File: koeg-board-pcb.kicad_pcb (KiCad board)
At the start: 2 copper layers, 10 parts, among them SW1 SW_Push_45deg, SW2 SW_Push_45deg, SW3 SW_Push_45deg, SW4 SW_Push_45deg, SW5 SW_Push_45deg, SW6 SW_Push_45deg, SW7 SW_Push_45deg, SW8 SW_Push_45deg, SW9 SW_Push_45deg, U1 STM32F730V8Tx

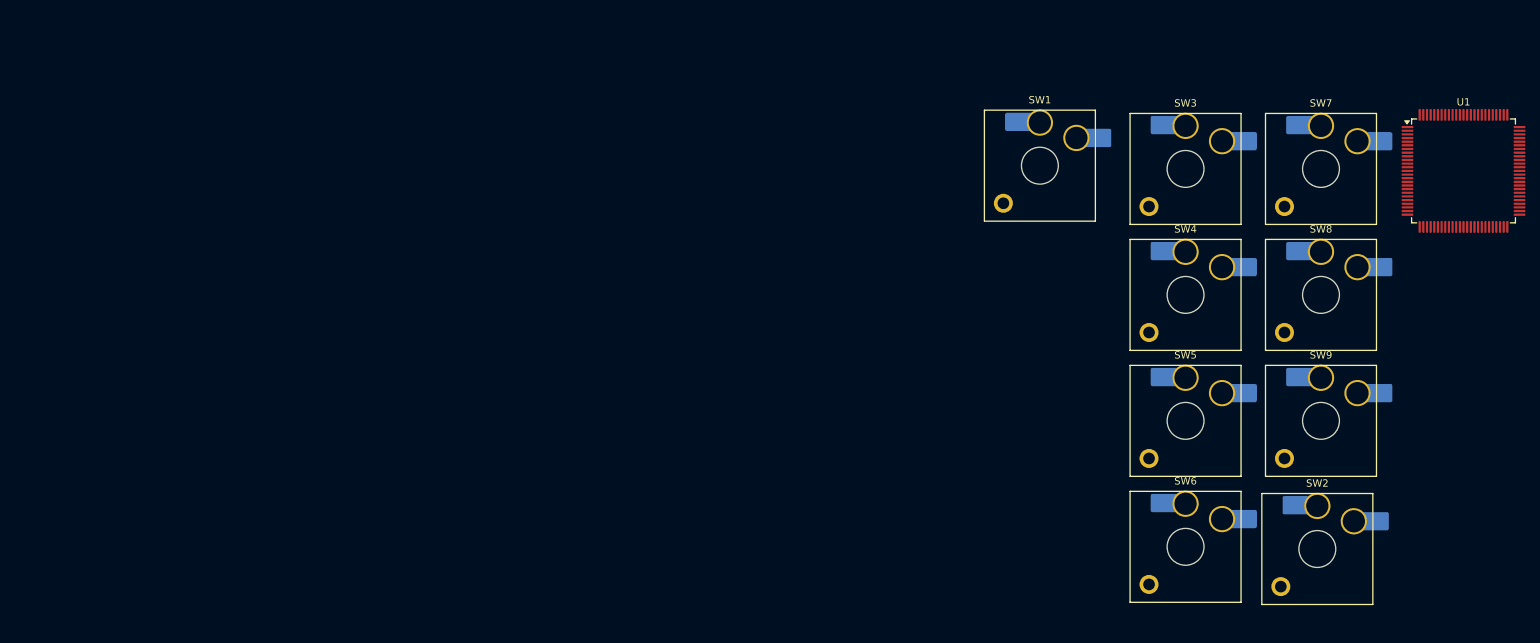
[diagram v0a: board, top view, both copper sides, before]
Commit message: before auto route
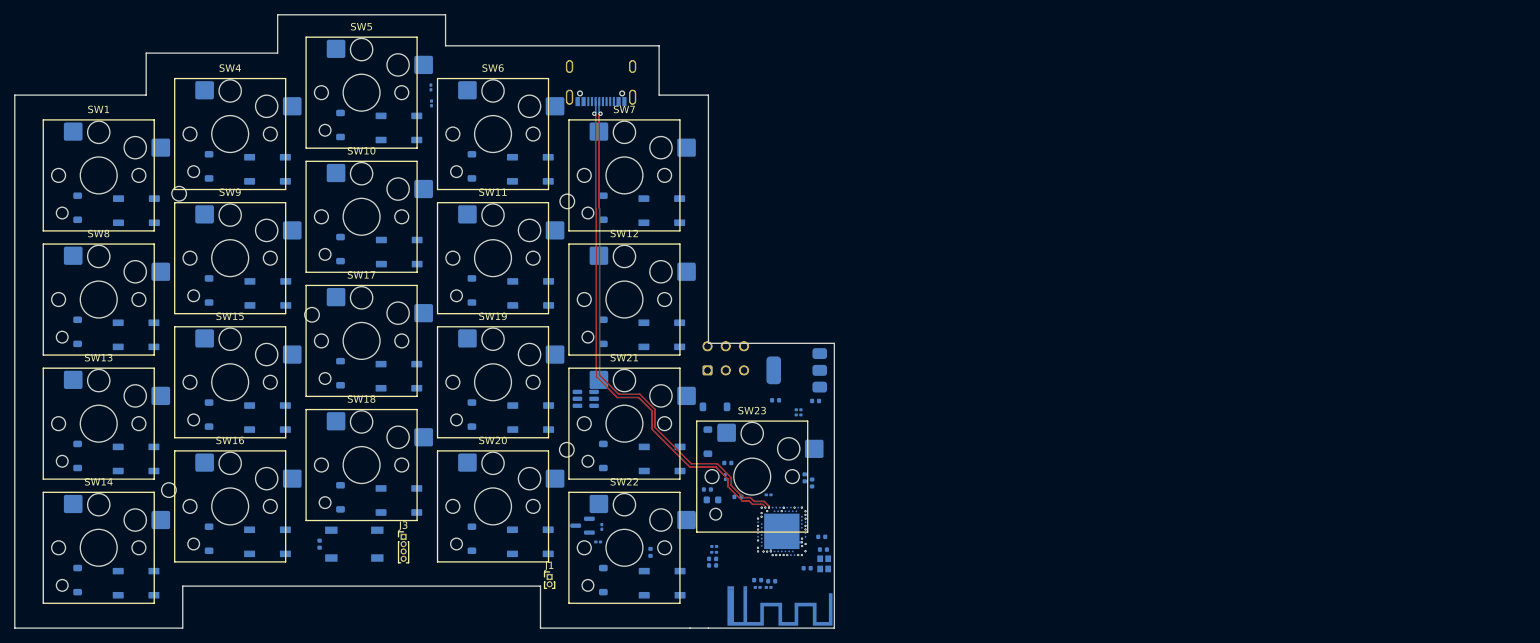
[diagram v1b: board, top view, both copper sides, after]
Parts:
- added AE1: PCB_Antenna, pcb_ant:pcb_antenna, B.Cu at (132.9, 122.5)
- added C1: 12pF, Capacitor_SMD:C_0402_1005Metric, B.Cu at (142.1, 119.5)
- added C10: 1pF, Capacitor_SMD:C_0402_1005Metric, B.Cu at (137.3, 121.3)
- added C11: 1.2pF, Capacitor_SMD:C_0402_1005Metric, B.Cu at (135.3, 121.1)
- added C12: 4.7uF, Capacitor_SMD:C_0402_1005Metric, B.Cu at (128.5, 108.7)
- added C13: 4.7uF, Capacitor_SMD:C_0402_1005Metric, B.Cu at (141.8, 107.1)
- added C14: 1uF, Capacitor_SMD:C_0402_1005Metric, B.Cu at (143.3, 96.6)
- added C15: 1uF, Capacitor_SMD:C_0402_1005Metric, B.Cu at (137.8, 96.5)
- added C16: 100nF, Capacitor_SMD:C_0402_1005Metric, B.Cu at (75.3, 116.2)
- added C2: 12pF, Capacitor_SMD:C_0402_1005Metric, B.Cu at (144.3, 116.9)
- added C3: 100nF, Capacitor_SMD:C_0402_1005Metric, B.Cu at (131.3, 105.1)
- added C4: 100pF, Capacitor_SMD:C_0402_1005Metric, B.Cu at (142.8, 107.8)
- added C5: 1uF, Capacitor_SMD:C_0402_1005Metric, B.Cu at (129.2, 119.1)
- added C6: 47nF, Capacitor_SMD:C_0402_1005Metric, B.Cu at (129.2, 118.2)
- added C7: 820pF, Capacitor_SMD:C_0402_1005Metric, B.Cu at (144.1, 115.2)
- added C8: 4.7uF, Capacitor_SMD:C_0402_1005Metric, B.Cu at (132.6, 109.7)
- added C9: 4.7uF, Capacitor_SMD:C_0402_1005Metric, B.Cu at (120.7, 117.3)
- added D1: 1N5819, Diode_SMD:D_SOD-123, B.Cu at (42.2, 70.1)
- added D10: 1N5819, Diode_SMD:D_SOD-123, B.Cu at (96.2, 81.4)
- added D11: 1N5819, Diode_SMD:D_SOD-123, B.Cu at (114.2, 87.1)
- added D12: 1N5819, Diode_SMD:D_SOD-123, B.Cu at (42.2, 104.1)
- added D13: 1N5819, Diode_SMD:D_SOD-123, B.Cu at (42.2, 121.1)
- added D14: 1N5819, Diode_SMD:D_SOD-123, B.Cu at (60.2, 98.4)
- added D15: 1N5819, Diode_SMD:D_SOD-123, B.Cu at (60.2, 115.4)
- added D16: 1N5819, Diode_SMD:D_SOD-123, B.Cu at (78.2, 92.8)
- added D17: 1N5819, Diode_SMD:D_SOD-123, B.Cu at (78.2, 109.8)
- added D18: 1N5819, Diode_SMD:D_SOD-123, B.Cu at (96.2, 98.4)
- added D19: 1N5819, Diode_SMD:D_SOD-123, B.Cu at (96.2, 115.4)
- added D2: 1N5819, Diode_SMD:D_SOD-123, B.Cu at (129.5, 97.4)
- added D20: 1N5819, Diode_SMD:D_SOD-123, B.Cu at (114.2, 104.1)
- added D21: 1N5819, Diode_SMD:D_SOD-123, B.Cu at (114.2, 121.1)
- added D22: 1N5819, Diode_SMD:D_SOD-123, B.Cu at (128.5, 102.1)
- added D23: WS2812B-2020, LED_SMD:LED_WS2812B_PLCC4_5.0x5.0mm_P3.2mm, B.Cu at (122.3, 121.5)
- added D24: WS2812B-2020, LED_SMD:LED_WS2812B_PLCC4_5.0x5.0mm_P3.2mm, B.Cu at (104.2, 115.9)
- added D25: WS2812B-2020, LED_SMD:LED_WS2812B_PLCC4_5.0x5.0mm_P3.2mm, B.Cu at (86.2, 110.2)
- added D26: WS2812B-2020, LED_SMD:LED_WS2812B_PLCC4_5.0x5.0mm_P3.2mm, B.Cu at (68.2, 115.9)
- added D27: WS2812B-2020, LED_SMD:LED_WS2812B_PLCC4_5.0x5.0mm_P3.2mm, B.Cu at (50.2, 121.5)
- added D28: WS2812B-2020, LED_SMD:LED_WS2812B_PLCC4_5.0x5.0mm_P3.2mm, B.Cu at (122.3, 104.5)
- added D29: WS2812B-2020, LED_SMD:LED_WS2812B_PLCC4_5.0x5.0mm_P3.2mm, B.Cu at (104.3, 98.8)
- added D3: 1N5819, Diode_SMD:D_SOD-123, B.Cu at (60.2, 64.4)
- added D30: WS2812B-2020, LED_SMD:LED_WS2812B_PLCC4_5.0x5.0mm_P3.2mm, B.Cu at (86.2, 93.2)
- added D31: WS2812B-2020, LED_SMD:LED_WS2812B_PLCC4_5.0x5.0mm_P3.2mm, B.Cu at (68.2, 98.8)
- added D32: WS2812B-2020, LED_SMD:LED_WS2812B_PLCC4_5.0x5.0mm_P3.2mm, B.Cu at (50.2, 104.5)
- added D33: WS2812B-2020, LED_SMD:LED_WS2812B_PLCC4_5.0x5.0mm_P3.2mm, B.Cu at (122.2, 87.5)
- added D34: WS2812B-2020, LED_SMD:LED_WS2812B_PLCC4_5.0x5.0mm_P3.2mm, B.Cu at (104.3, 81.8)
- added D35: WS2812B-2020, LED_SMD:LED_WS2812B_PLCC4_5.0x5.0mm_P3.2mm, B.Cu at (86.3, 76.2)
- added D36: WS2812B-2020, LED_SMD:LED_WS2812B_PLCC4_5.0x5.0mm_P3.2mm, B.Cu at (68.3, 81.8)
- added D37: WS2812B-2020, LED_SMD:LED_WS2812B_PLCC4_5.0x5.0mm_P3.2mm, B.Cu at (50.2, 87.5)
- added D38: WS2812B-2020, LED_SMD:LED_WS2812B_PLCC4_5.0x5.0mm_P3.2mm, B.Cu at (122.2, 70.5)
- added D39: WS2812B-2020, LED_SMD:LED_WS2812B_PLCC4_5.0x5.0mm_P3.2mm, B.Cu at (104.2, 64.8)
- added D4: 1N5819, Diode_SMD:D_SOD-123, B.Cu at (78.2, 58.8)
- added D40: WS2812B-2020, LED_SMD:LED_WS2812B_PLCC4_5.0x5.0mm_P3.2mm, B.Cu at (86.2, 59.2)
- added D41: WS2812B-2020, LED_SMD:LED_WS2812B_PLCC4_5.0x5.0mm_P3.2mm, B.Cu at (68.2, 64.8)
- added D42: WS2812B-2020, LED_SMD:LED_WS2812B_PLCC4_5.0x5.0mm_P3.2mm, B.Cu at (50.3, 70.5)
- added D5: 1N5819, Diode_SMD:D_SOD-123, B.Cu at (96.2, 64.4)
- added D6: 1N5819, Diode_SMD:D_SOD-123, B.Cu at (114.2, 70.1)
- added D7: 1N5819, Diode_SMD:D_SOD-123, B.Cu at (42.2, 87.1)
- added D8: 1N5819, Diode_SMD:D_SOD-123, B.Cu at (60.2, 81.4)
- added D9: 1N5819, Diode_SMD:D_SOD-123, B.Cu at (78.2, 75.8)
- added F1: 500mA, Fuse:Fuse_0603_1608Metric, B.Cu at (129.2, 110.1)
- added H1: MountingHole, MountingHole:MountingHole_2mm, B.Cu at (56.1, 68.2)
- added H2: MountingHole, MountingHole:MountingHole_2mm, B.Cu at (74.3, 84.8)
- added H3: MountingHole, MountingHole:MountingHole_2mm, B.Cu at (109.2, 103.3)
- added H4: MountingHole, MountingHole:MountingHole_2mm, B.Cu at (54.7, 108.8)
- added H5: MountingHole, MountingHole:MountingHole_2mm, B.Cu at (109.3, 69.2)
- added J1: Conn_01x02, Connector_PinHeader_1.00mm:PinHeader_1x02_P1.00mm_Vertical, F.Cu at (106.8, 120.7)
- added J2: USB_C_Receptacle_USB2.0_14P, Connector_USB:USB_C_Receptacle_G-Switch_GT-USB-7010ASV, B.Cu at (113.9, 51.8)
- added J3: SWD_Connector, Connector_PinHeader_1.00mm:PinHeader_1x04_P1.00mm_Vertical, F.Cu at (86.8, 115.2)
- added L1: 10uH, Inductor_SMD:L_0201_0603Metric, B.Cu at (129.4, 116.5)
- added L2: 15nH, Inductor_SMD:L_0201_0603Metric, B.Cu at (129.4, 117.3)
- added L3: 10uH, Inductor_SMD:L_0201_0603Metric, B.Cu at (130.9, 107.0)
- added L4: 4.7nH, Inductor_SMD:L_0201_0603Metric, B.Cu at (136.8, 122.1)
- added L5: 2.2nH, Inductor_SMD:L_0201_0603Metric, B.Cu at (135.3, 122.1)
- added Q1: BSS138, Package_TO_SOT_SMD:SOT-23, B.Cu at (111.4, 113.7)
- added R1: 5.1k, Resistor_SMD:R_0201_0603Metric, B.Cu at (90.6, 53.6)
- added R2: 5.1k, Resistor_SMD:R_0201_0603Metric, B.Cu at (90.7, 55.8)
- added R3: 2M, Resistor_SMD:R_0201_0603Metric, B.Cu at (140.9, 98.5)
- added R4: 810K, Resistor_SMD:R_0201_0603Metric, B.Cu at (141.0, 97.8)
- added R5: 10K, Resistor_SMD:R_0201_0603Metric, B.Cu at (114.0, 113.8)
- added R6: 10K, Resistor_SMD:R_0201_0603Metric, B.Cu at (113.5, 115.9)
- added R7: 100K, Resistor_SMD:R_0201_0603Metric, B.Cu at (136.8, 109.4)
- added SW10: SW_Push, PCM_Switch_Keyboard_Hotswap_Kailh:SW_Hotswap_Kailh_Choc_V1V2_1.00u, F.Cu at (81.1, 71.3)
- added SW11: SW_Push, PCM_Switch_Keyboard_Hotswap_Kailh:SW_Hotswap_Kailh_Choc_V1V2_1.00u, F.Cu at (99.1, 77.0)
- added SW12: SW_Push, PCM_Switch_Keyboard_Hotswap_Kailh:SW_Hotswap_Kailh_Choc_V1V2_1.00u, F.Cu at (117.1, 82.7)
- added SW13: SW_Push, PCM_Switch_Keyboard_Hotswap_Kailh:SW_Hotswap_Kailh_Choc_V1V2_1.00u, F.Cu at (45.1, 99.7)
- added SW14: SW_Push, PCM_Switch_Keyboard_Hotswap_Kailh:SW_Hotswap_Kailh_Choc_V1V2_1.00u, F.Cu at (45.1, 116.7)
- added SW15: SW_Push, PCM_Switch_Keyboard_Hotswap_Kailh:SW_Hotswap_Kailh_Choc_V1V2_1.00u, F.Cu at (63.1, 94.0)
- added SW16: SW_Push, PCM_Switch_Keyboard_Hotswap_Kailh:SW_Hotswap_Kailh_Choc_V1V2_1.00u, F.Cu at (63.1, 111.0)
- added SW17: SW_Push, PCM_Switch_Keyboard_Hotswap_Kailh:SW_Hotswap_Kailh_Choc_V1V2_1.00u, F.Cu at (81.1, 88.3)
- added SW18: SW_Push, PCM_Switch_Keyboard_Hotswap_Kailh:SW_Hotswap_Kailh_Choc_V1V2_1.00u, F.Cu at (81.1, 105.3)
- added SW19: SW_Push, PCM_Switch_Keyboard_Hotswap_Kailh:SW_Hotswap_Kailh_Choc_V1V2_1.00u, F.Cu at (99.1, 94.0)
- added SW20: SW_Push, PCM_Switch_Keyboard_Hotswap_Kailh:SW_Hotswap_Kailh_Choc_V1V2_1.00u, F.Cu at (99.1, 111.0)
- added SW21: SW_Push, PCM_Switch_Keyboard_Hotswap_Kailh:SW_Hotswap_Kailh_Choc_V1V2_1.00u, F.Cu at (117.1, 99.7)
- added SW22: SW_Push, PCM_Switch_Keyboard_Hotswap_Kailh:SW_Hotswap_Kailh_Choc_V1V2_1.00u, F.Cu at (117.1, 116.7)
- added SW23: SW_Push, PCM_Switch_Keyboard_Hotswap_Kailh:SW_Hotswap_Kailh_Choc_V1V2_1.75u_90deg, F.Cu at (134.6, 106.9)
- added U2: AMS1117-5.0, Package_TO_SOT_SMD:SOT-223-3_TabPin2, B.Cu at (140.7, 92.4)
- added U3: USBLC6-2SC6, Package_TO_SOT_SMD:SOT-23-6, B.Cu at (111.8, 96.3)
- added Y1: Crystal_GND2, Crystal:Crystal_SMD_2016-4Pin_2.0x1.6mm, B.Cu at (144.4, 118.9)
- SW1, SW4, SW5, SW6, SW7, SW8, SW9: value SW_Push_45deg -> SW_Push; footprint PCM_Switch_Keyboard_Hotswap_Kailh:SW_Hotswap_Kailh_Choc_V2_Plated -> PCM_Switch_Keyboard_Hotswap_Kailh:SW_Hotswap_Kailh_Choc_V1V2_1.00u
- SW2: value SW_Push_45deg -> Reset Button; footprint PCM_Switch_Keyboard_Hotswap_Kailh:SW_Hotswap_Kailh_Choc_V2_Plated -> Button_Switch_SMD:SW_SPST_TL3342; moved to B.Cu
- SW3: value SW_Push_45deg -> SW_On_Off; footprint PCM_Switch_Keyboard_Hotswap_Kailh:SW_Hotswap_Kailh_Choc_V2_Plated -> Button_Switch_THT:SW_CK_JS202011AQN_DPDT_Angled; moved to B.Cu
- U1: value STM32F730V8Tx -> nRF52840; footprint Package_QFP:LQFP-100_14x14mm_P0.5mm -> Package_DFN_QFN:Nordic_AQFN-73-1EP_7x7mm_P0.5mm; moved to B.Cu
- moved SW8 167.4 mm to (45.1, 82.7)
- moved SW9 151.1 mm to (63.1, 77.0)
- moved SW4 132.7 mm to (63.1, 60.0)
- moved SW2 131.9 mm to (80.1, 116.2), turned to 180 degrees
- moved SW1 128.9 mm to (45.1, 65.7)
- moved SW5 121.5 mm to (81.1, 54.3)
- moved SW6 110.4 mm to (99.1, 60.0)
- moved U1 105.6 mm to (138.7, 114.4)
- moved SW7 95.4 mm to (117.1, 65.7)
- moved SW3 71.0 mm to (128.5, 92.4)
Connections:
- SW1 pad 1: unconnected-(SW1-Pad1) -> Net-(D1-A)
- SW1 pad 2: GND -> /COL0
- SW2 pad 1: unconnected-(SW2-Pad1) -> /RESET
- SW3 pad 2: GND -> VBAT
- SW4 pad 1: unconnected-(SW4-Pad1) -> Net-(D3-A)
- SW4 pad 2: GND -> /COL1
- SW5 pad 1: unconnected-(SW5-Pad1) -> Net-(D4-A)
- SW5 pad 2: GND -> /COL2
- SW6 pad 1: unconnected-(SW6-Pad1) -> Net-(D5-A)
- SW6 pad 2: GND -> /COL3
- SW7 pad 1: unconnected-(SW7-Pad1) -> Net-(D6-A)
- SW7 pad 2: GND -> /COL4
- SW8 pad 1: unconnected-(SW8-Pad1) -> Net-(D7-A)
- SW8 pad 2: GND -> /COL0
- SW9 pad 1: unconnected-(SW9-Pad1) -> Net-(D8-A)
- SW9 pad 2: GND -> /COL1
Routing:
- net /D-: track 0.00 -> 70.6 mm, vias 0 -> 2
- net /D+: track 0.00 -> 70.6 mm, vias 0 -> 2
- net GND: track 0.00 -> 6.74 mm, vias 0 -> 2
- net /DEC3: track 0.00 -> 0.11 mm, vias 0 -> 1
- net /DEC4: track 0.00 -> 0.05 mm, vias 0 -> 2
- net V_SYS: track 0.00 -> 0.04 mm, vias 0 -> 5
- net /XC1: track 0.00 -> 0.03 mm, vias 0 -> 1
- net /RESET: track 0.00 -> 0.03 mm, vias 0 -> 1
- net 3.2V-5V: track 0.00 -> 0.03 mm, vias 0 -> 1
- net /ANT: track 0.00 -> 0.03 mm, vias 0 -> 1
- net /DECUSB: track 0.00 -> 0.03 mm, vias 0 -> 1
- net /DCC: track 0.00 -> 0.02 mm, vias 0 -> 1
- net /DCCH: track 0.00 -> 0.02 mm, vias 0 -> 1
- net /ROW0: track 0.00 -> 0.02 mm, vias 0 -> 1
- net LED_PIN: track 0.00 -> 0.01 mm, vias 0 -> 1
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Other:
- board outline added: 112.2 x 84 mm

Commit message: autorouted
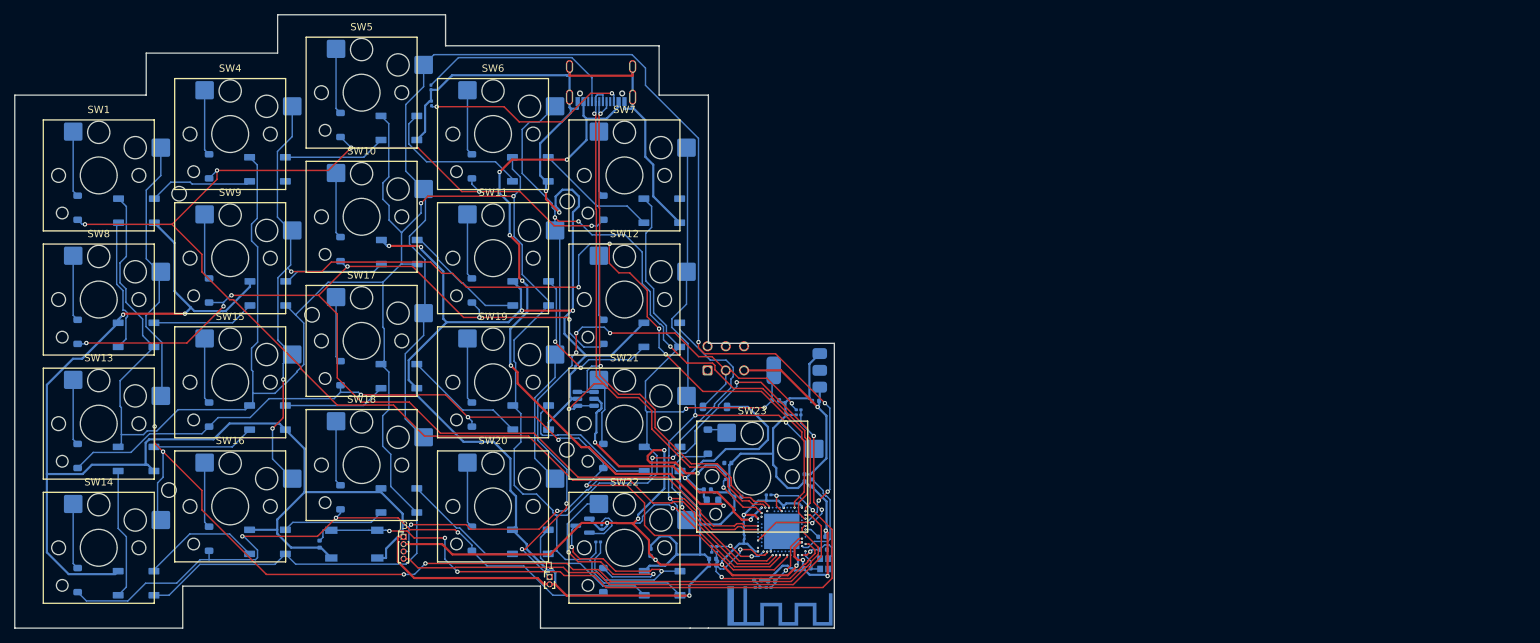
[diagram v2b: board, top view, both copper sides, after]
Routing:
- net GND: track 6.74 -> 581.3 mm, vias 2 -> 14
- net LED_5V: track 0.00 -> 420.4 mm, vias 0 -> 4
- net /ROW0: track 0.02 -> 191.6 mm, vias 1 -> 6
- net /COL2: track 0.00 -> 168.6 mm, vias 0 -> 4
- net /ROW1: track 0.01 -> 167.1 mm, vias 1 -> 7
- net /COL0: track 0.00 -> 162.4 mm, vias 1 -> 5
- net /COL1: track 0.00 -> 161.2 mm, vias 1 -> 8
- net /COL3: track 0.01 -> 123.6 mm, vias 1 -> 4
- net /ROW2: track 0.00 -> 122.1 mm, vias 1 -> 5
- net V_SYS: track 0.04 -> 118.1 mm, vias 5 -> 13
- net /RESET: track 0.03 -> 96.3 mm, vias 1 -> 6
- net VBUS: track 0.00 -> 93.1 mm, vias 0 -> 6
- net /ROW3: track 0.01 -> 89.6 mm, vias 1 -> 4
- net /COL4: track 0.00 -> 88.5 mm, vias 1 -> 4
- net /SWDIO: track 0.00 -> 84.7 mm, vias 1 -> 6
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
